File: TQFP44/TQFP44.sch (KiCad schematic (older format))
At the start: 6 parts, among them J1 Conn_01x22, J2 Conn_01x22, J3 Conn_02x22_Counter_Clockwise, J4 Conn_02x22_Counter_Clockwise_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, J5 Conn_02x22_Counter_Clockwise, J6 Conn_01x06

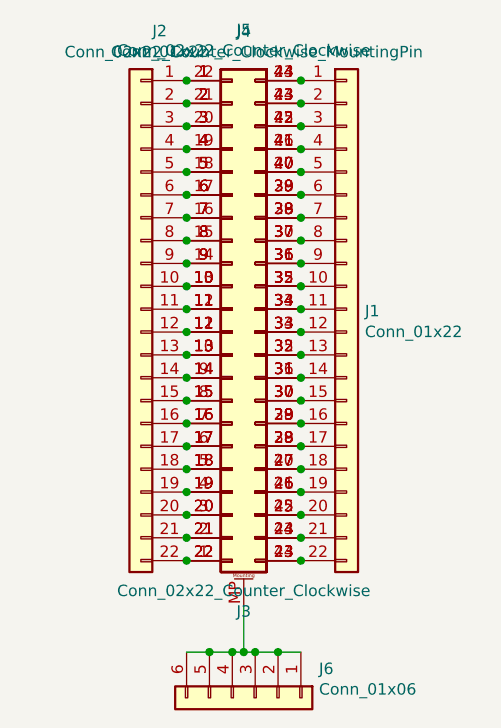
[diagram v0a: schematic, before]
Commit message: Final Revisions
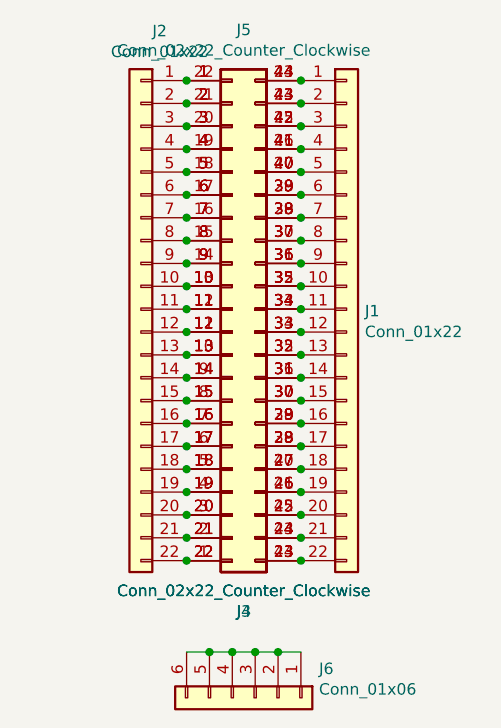
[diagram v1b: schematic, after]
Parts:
- removed J4: Conn_02x22_Counter_Clockwise_MountingPin, Package_DFN_QFN:QFN-44-1EP_7x7mm_P0.5mm_EP5.2x5.2mm, symbol Connector_Generic_MountingPin:Conn_02x22_Counter_Clockwise_MountingPin
- added J4: Conn_02x22_Counter_Clockwise, Package_DFN_QFN:QFN-44-1EP_7x7mm_P0.5mm_EP5.15x5.15mm, symbol Connector_Generic:Conn_02x22_Counter_Clockwise
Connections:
- net at J1.1 (Pin_1), J3.44 (Pin_44), J5.23 (Pin_23): now also J4.44 (Pin_44)
- net at J1.10 (Pin_10), J3.35 (Pin_35), J5.32 (Pin_32): now also J4.35 (Pin_35)
- net at J1.11 (Pin_11), J3.34 (Pin_34), J5.33 (Pin_33): now also J4.34 (Pin_34)
- net at J1.12 (Pin_12), J3.33 (Pin_33), J5.34 (Pin_34): now also J4.33 (Pin_33)
- net at J1.13 (Pin_13), J3.32 (Pin_32), J5.35 (Pin_35): now also J4.32 (Pin_32)
- net at J1.14 (Pin_14), J3.31 (Pin_31), J5.36 (Pin_36): now also J4.31 (Pin_31)
- net at J1.15 (Pin_15), J3.30 (Pin_30), J5.37 (Pin_37): now also J4.30 (Pin_30)
- net at J1.16 (Pin_16), J3.29 (Pin_29), J5.38 (Pin_38): now also J4.29 (Pin_29)
- net at J1.17 (Pin_17), J3.28 (Pin_28), J5.39 (Pin_39): now also J4.28 (Pin_28)
- net at J1.18 (Pin_18), J3.27 (Pin_27), J5.40 (Pin_40): now also J4.27 (Pin_27)
- net at J1.19 (Pin_19), J3.26 (Pin_26), J5.41 (Pin_41): now also J4.26 (Pin_26)
- net at J1.2 (Pin_2), J3.43 (Pin_43), J5.24 (Pin_24): now also J4.43 (Pin_43)
- net at J1.20 (Pin_20), J3.25 (Pin_25), J5.42 (Pin_42): now also J4.25 (Pin_25)
- net at J1.21 (Pin_21), J3.24 (Pin_24), J5.43 (Pin_43): now also J4.24 (Pin_24)
- net at J1.22 (Pin_22), J3.23 (Pin_23), J5.44 (Pin_44): now also J4.23 (Pin_23)
- net at J1.3 (Pin_3), J3.42 (Pin_42), J5.25 (Pin_25): now also J4.42 (Pin_42)
- net at J1.4 (Pin_4), J3.41 (Pin_41), J5.26 (Pin_26): now also J4.41 (Pin_41)
- net at J1.5 (Pin_5), J3.40 (Pin_40), J5.27 (Pin_27): now also J4.40 (Pin_40)
- net at J1.6 (Pin_6), J3.39 (Pin_39), J5.28 (Pin_28): now also J4.39 (Pin_39)
- net at J1.7 (Pin_7), J3.38 (Pin_38), J5.29 (Pin_29): now also J4.38 (Pin_38)
- net at J1.8 (Pin_8), J3.37 (Pin_37), J5.30 (Pin_30): now also J4.37 (Pin_37)
- net at J1.9 (Pin_9), J3.36 (Pin_36), J5.31 (Pin_31): now also J4.36 (Pin_36)
- net at J2.1 (Pin_1), J3.1 (Pin_1), J5.22 (Pin_22): now also J4.1 (Pin_1)
- net at J2.10 (Pin_10), J3.10 (Pin_10), J5.13 (Pin_13): now also J4.10 (Pin_10)
- net at J2.11 (Pin_11), J3.11 (Pin_11), J5.12 (Pin_12): now also J4.11 (Pin_11)
- net at J2.12 (Pin_12), J3.12 (Pin_12), J5.11 (Pin_11): now also J4.12 (Pin_12)
- net at J2.13 (Pin_13), J3.13 (Pin_13), J5.10 (Pin_10): now also J4.13 (Pin_13)
- net at J2.14 (Pin_14), J3.14 (Pin_14), J5.9 (Pin_9): now also J4.14 (Pin_14)
- net at J2.15 (Pin_15), J3.15 (Pin_15), J5.8 (Pin_8): now also J4.15 (Pin_15)
- net at J2.16 (Pin_16), J3.16 (Pin_16), J5.7 (Pin_7): now also J4.16 (Pin_16)
- net at J2.17 (Pin_17), J3.17 (Pin_17), J5.6 (Pin_6): now also J4.17 (Pin_17)
- net at J2.18 (Pin_18), J3.18 (Pin_18), J5.5 (Pin_5): now also J4.18 (Pin_18)
- net at J2.19 (Pin_19), J3.19 (Pin_19), J5.4 (Pin_4): now also J4.19 (Pin_19)
- net at J2.2 (Pin_2), J3.2 (Pin_2), J5.21 (Pin_21): now also J4.2 (Pin_2)
- net at J2.20 (Pin_20), J3.20 (Pin_20), J5.3 (Pin_3): now also J4.20 (Pin_20)
- net at J2.21 (Pin_21), J3.21 (Pin_21), J5.2 (Pin_2): now also J4.21 (Pin_21)
- net at J2.22 (Pin_22), J3.22 (Pin_22), J5.1 (Pin_1): now also J4.22 (Pin_22)
- net at J2.3 (Pin_3), J3.3 (Pin_3), J5.20 (Pin_20): now also J4.3 (Pin_3)
- net at J2.4 (Pin_4), J3.4 (Pin_4), J5.19 (Pin_19): now also J4.4 (Pin_4)
- net at J2.5 (Pin_5), J3.5 (Pin_5), J5.18 (Pin_18): now also J4.5 (Pin_5)
- net at J2.6 (Pin_6), J3.6 (Pin_6), J5.17 (Pin_17): now also J4.6 (Pin_6)
- net at J2.7 (Pin_7), J3.7 (Pin_7), J5.16 (Pin_16): now also J4.7 (Pin_7)
- net at J2.8 (Pin_8), J3.8 (Pin_8), J5.15 (Pin_15): now also J4.8 (Pin_8)
- net at J2.9 (Pin_9), J3.9 (Pin_9), J5.14 (Pin_14): now also J4.9 (Pin_9)
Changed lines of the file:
@@
-	1    0    0    -1
-$EndComp
-$Comp
-L Connector_Generic_MountingPin:Conn_02x22_Counter_Clockwise_MountingPin J4
-U 1 1 5D32F516
-P 5300 3850
-F 0 "J4" H 5350 5065 50  0000 C CNN
-F 1 "Conn_02x22_Counter_Clockwise_MountingPin" H 5350 4975 50  0000 C CNN
-F 2 "Package_DFN_QFN:QFN-44-1EP_7x7mm_P0.5mm_EP5.2x5.2mm" H 5300 3850 50  0001 C CNN
-F 3 "~" H 5300 3850 50  0001 C CNN
-	1    5300 3850
 	1    0    0    -1
 $EndComp
@@
 	0    1    1    0
 $EndComp
-Wire Wire Line
-	5350 5150 5350 5350
-Wire Wire Line
-	5350 5350 5400 5350
 Connection ~ 5400 5350
 Wire Wire Line
@@
 Wire Wire Line
 	5100 5350 5200 5350
-Connection ~ 5350 5350
 Connection ~ 5200 5350
 Wire Wire Line
@@
 Connection ~ 5300 5350
 Wire Wire Line
-	5300 5350 5350 5350
+	5300 5350 5400 5350
+$Comp
+L Connector_Generic:Conn_02x22_Counter_Clockwise J4
+U 1 1 5D472302
+P 5300 3850
+F 0 "J4" H 5350 2528 50  0000 C CNN
+F 1 "Conn_02x22_Counter_Clockwise" H 5350 2618 50  0000 C CNN
+F 2 "Package_DFN_QFN:QFN-44-1EP_7x7mm_P0.5mm_EP5.15x5.15mm" H 5300 3850 50  0001 C CNN
+F 3 "~" H 5300 3850 50  0001 C CNN
+	1    5300 3850
+	1    0    0    -1
+$EndComp
 $EndSCHEMATC
